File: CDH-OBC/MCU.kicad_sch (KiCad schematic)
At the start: 23 parts, among them J5 Conn_ARM_JTAG_SWD_20, J6 UART, U1 TMS5700714APZQQ1

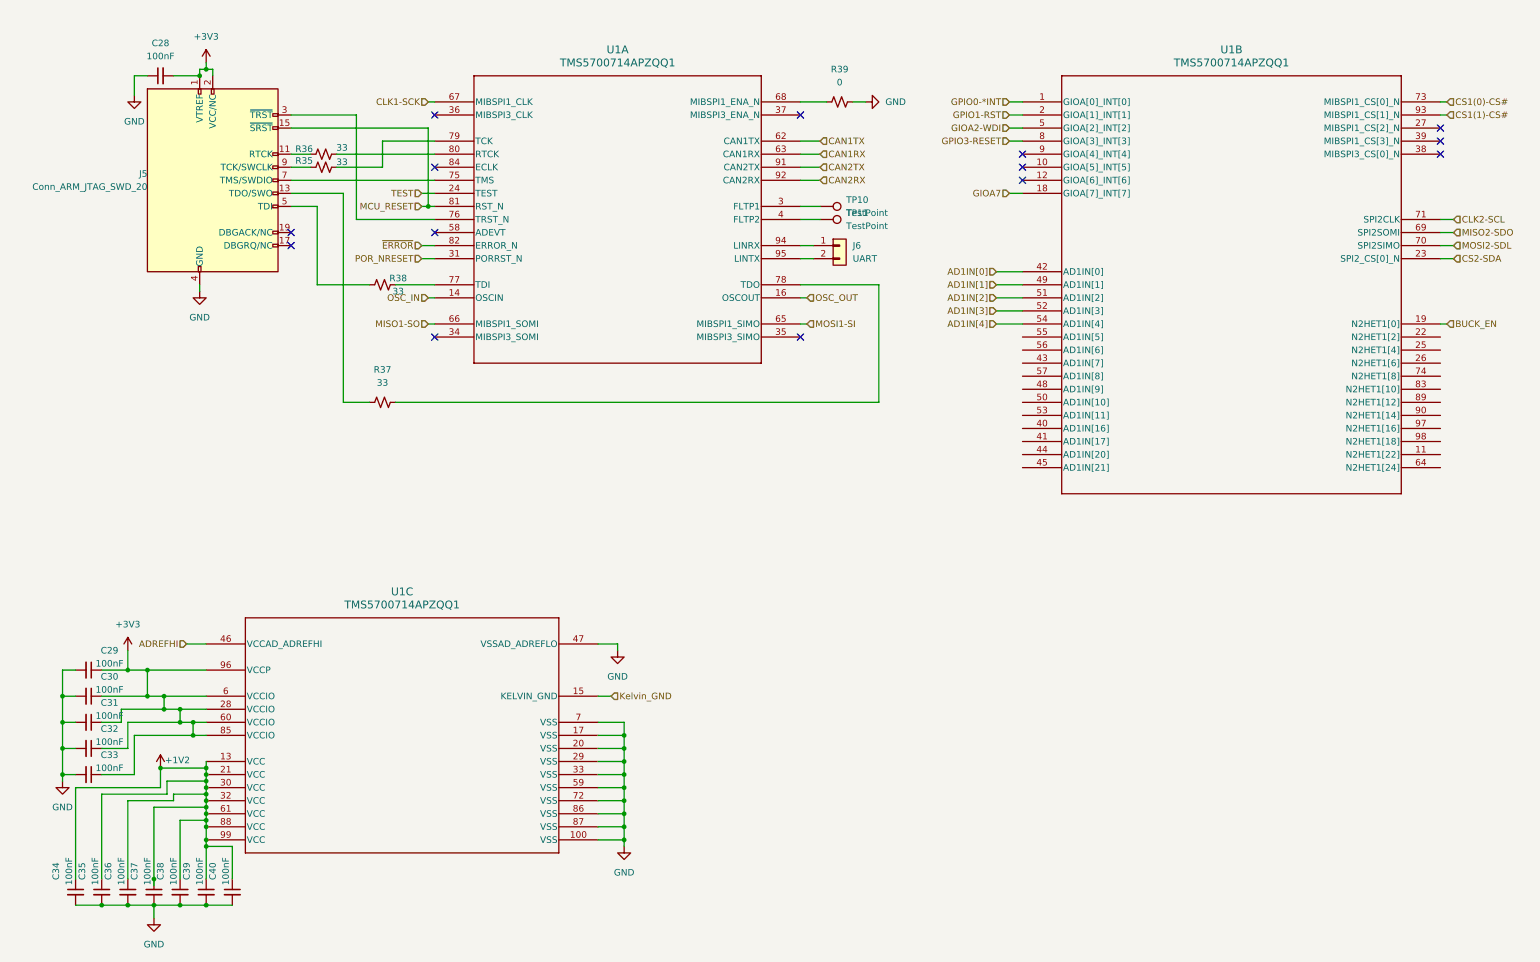
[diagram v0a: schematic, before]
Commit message: finished schematic
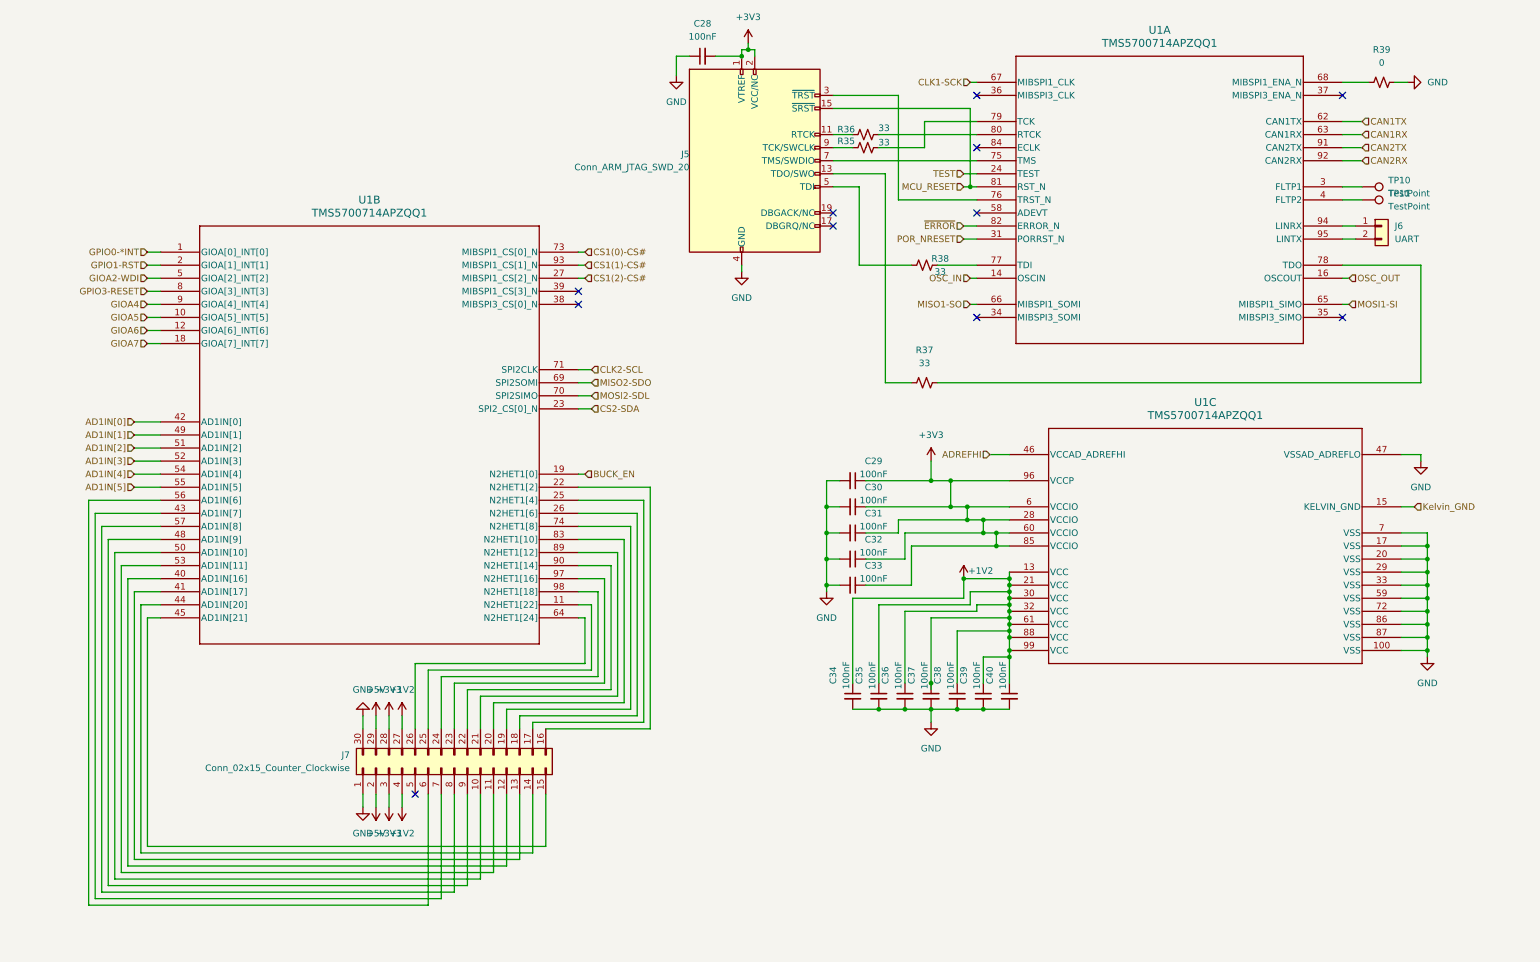
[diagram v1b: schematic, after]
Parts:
- added J7: Conn_02x15_Counter_Clockwise, Connector_PinHeader_2.54mm:PinHeader_2x15_P2.54mm_Vertical, symbol Connector_Generic:Conn_02x15_Counter_Clockwise
- C28, C29, C30, C31, C32, C33, C34, C35, C36, C37, C38, C39, C40: footprint (none) -> Capacitor_SMD:C_0603_1608Metric
- J5: footprint (none) -> Connector_PinHeader_2.54mm:PinHeader_2x10_P2.54mm_Vertical
- J6: footprint (none) -> Connector_PinHeader_2.54mm:PinHeader_1x02_P2.54mm_Vertical
- R35, R36, R37, R38, R39: footprint (none) -> Resistor_SMD:R_0603_1608Metric
- TP10, TP11: footprint (none) -> TestPoint:TestPoint_Pad_D1.0mm
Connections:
- net +1V2: now also J7.27 (Pin_27), J7.4 (Pin_4)
- net +3V3: now also J7.28 (Pin_28), J7.3 (Pin_3)
- net GND: now also J7.1 (Pin_1), J7.30 (Pin_30)
- net GIOA5: now reaches U1.10 (GIOA[5]_INT[5])
- net at U1.11 (N2HET1[22]): now also J7.25 (Pin_25)
- net GIOA6: now reaches U1.12 (GIOA[6]_INT[6])
- net at U1.22 (N2HET1[2]): now also J7.16 (Pin_16)
- net at U1.25 (N2HET1[4]): now also J7.17 (Pin_17)
- net at U1.26 (N2HET1[6]): now also J7.18 (Pin_18)
- net CS1(2)-CS#: now reaches U1.27 (MIBSPI1_CS[2]_N)
- net at U1.40 (AD1IN[16]): now also J7.12 (Pin_12)
- net at U1.41 (AD1IN[17]): now also J7.13 (Pin_13)
- net at U1.43 (AD1IN[7]): now also J7.7 (Pin_7)
- net at U1.44 (AD1IN[20]): now also J7.14 (Pin_14)
- net at U1.45 (AD1IN[21]): now also J7.15 (Pin_15)
- net at U1.48 (AD1IN[9]): now also J7.9 (Pin_9)
- net at U1.50 (AD1IN[10]): now also J7.10 (Pin_10)
- net at U1.53 (AD1IN[11]): now also J7.11 (Pin_11)
- net AD1IN[5]: now reaches U1.55 (AD1IN[5])
- net at U1.56 (AD1IN[6]): now also J7.6 (Pin_6)
- net at U1.57 (AD1IN[8]): now also J7.8 (Pin_8)
- net at U1.64 (N2HET1[24]): now also J7.26 (Pin_26)
- net at U1.74 (N2HET1[8]): now also J7.19 (Pin_19)
- net at U1.83 (N2HET1[10]): now also J7.20 (Pin_20)
- net at U1.89 (N2HET1[12]): now also J7.21 (Pin_21)
- net GIOA4: now reaches U1.9 (GIOA[4]_INT[4])
- net at U1.90 (N2HET1[14]): now also J7.22 (Pin_22)
- net at U1.97 (N2HET1[16]): now also J7.23 (Pin_23)
- net at U1.98 (N2HET1[18]): now also J7.24 (Pin_24)
- new net +5V: J7.2 (Pin_2), J7.29 (Pin_29)
- no-connect marks 14 -> 11
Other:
- moved on the sheet: C28, C29, C30, C31, C32, C33, C34, C35, C36, C37, C38, C39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
